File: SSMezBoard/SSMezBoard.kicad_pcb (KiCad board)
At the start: 2 copper layers, 2 parts, among them U1 DFRobot_DC_Controller

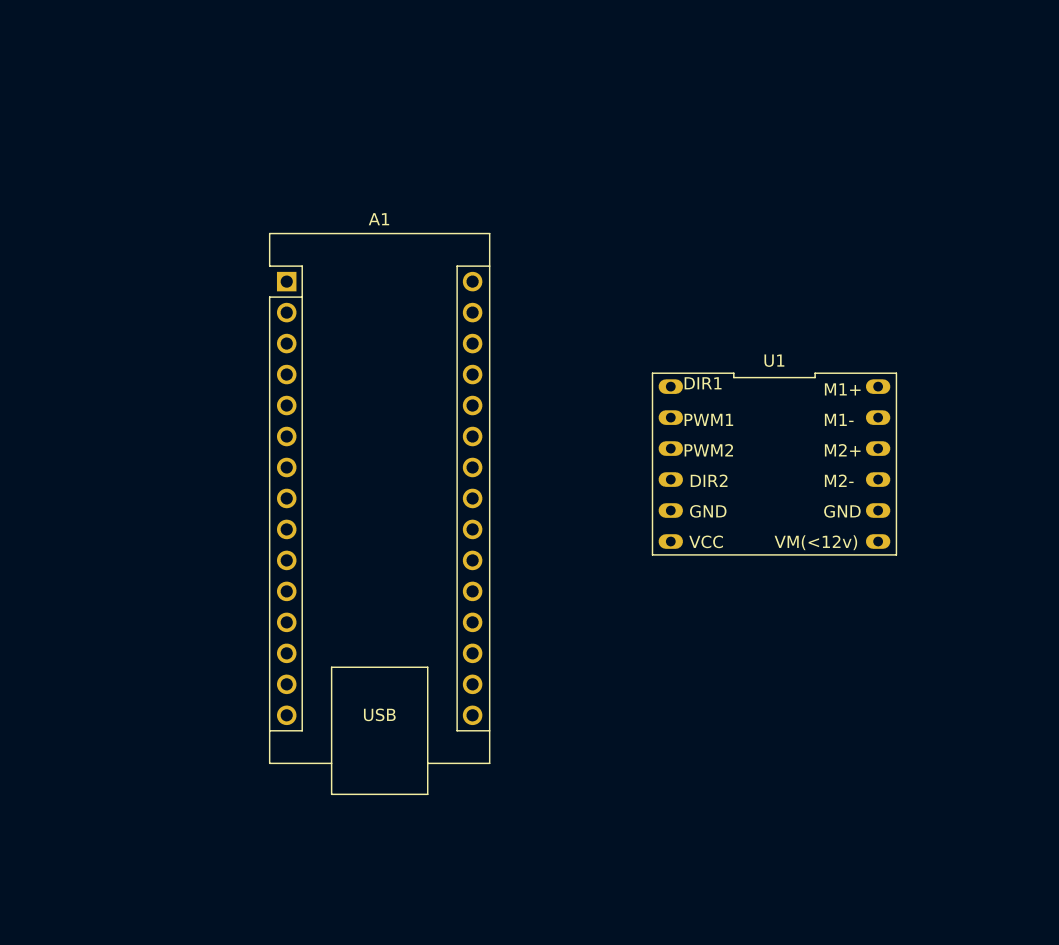
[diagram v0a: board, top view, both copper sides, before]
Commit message: Sort of ready for JLCPCB
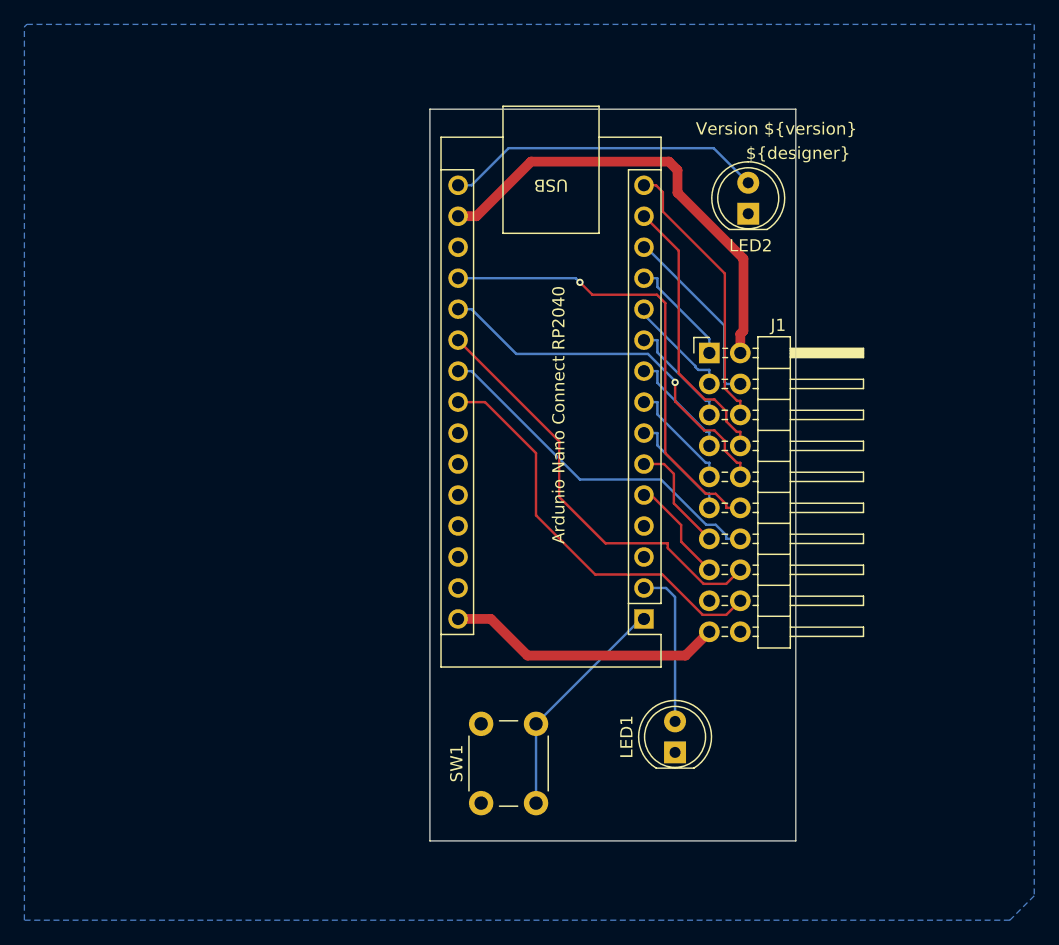
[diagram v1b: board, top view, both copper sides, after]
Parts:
- removed U1: DFRobot_DC_Controller, PBFootPrintLibrary:DFRobot_DC_Controller
- added J1: Conn_02x10_Odd_Even, Connector_PinHeader_2.54mm:PinHeader_2x10_P2.54mm_Horizontal, F.Cu at (162.9, 75.8)
- added LED1: LED, LED_THT:LED_D5.0mm, F.Cu at (160.1, 108.5)
- added LED2: LED, LED_THT:LED_D5.0mm, F.Cu at (166.1, 64.4)
- added SW1: TACT_SW, Button_Switch_THT:SW_PUSH_6mm, F.Cu at (144.2, 112.7)
- moved A1 40.3 mm to (157.6, 97.6), turned to 180 degrees
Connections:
- net Net-(A1-GND-Pad29) renamed GND
- A1 pad 1: unconnected-(A1-D1/TX-Pad1) -> Net-(A1-D1/TX)
- A1 pad 10: unconnected-(A1-D7-Pad10) -> RIGHT_ENC_B
- A1 pad 11: unconnected-(A1-D8-Pad11) -> LEFT_ENC_A
- A1 pad 12: unconnected-(A1-D9-Pad12) -> LEFT_ENC_B
- A1 pad 13: unconnected-(A1-D10/CS-Pad13) -> SENSOR_LED
- A1 pad 14: unconnected-(A1-D11/COPI-Pad14) -> GPIO_DIAG
- A1 pad 15: unconnected-(A1-D12/CIPO-Pad15) -> GPIO_FRONT
- A1 pad 16: unconnected-(A1-D13/SCK-Pad16) -> Net-(A1-D13/SCK)
- A1 pad 17: Net-(A1-3V3) -> Vcc
- A1 pad 19: unconnected-(A1-A0-Pad19) -> RIGHT_DIAG_ADC
- A1 pad 2: unconnected-(A1-D0/RX-Pad2) -> Net-(A1-D0/RX)
- A1 pad 20: unconnected-(A1-A1-Pad20) -> RIGHT_FRONT_ADC
- A1 pad 21: unconnected-(A1-A2-Pad21) -> LEFT_FRONT_ADC
- A1 pad 22: unconnected-(A1-A3-Pad22) -> LEFT_DIAG_ADC
- A1 pad 23: unconnected-(A1-SDA/A4-Pad23) -> GPIO12_D18
- A1 pad 30: unconnected-(A1-VIN-Pad30) -> Vbatt
- A1 pad 5: unconnected-(A1-D2-Pad5) -> RIGHT_Motor_PWM
- A1 pad 6: unconnected-(A1-D3-Pad6) -> LEFT_Motor_PWM
- A1 pad 7: unconnected-(A1-D4-Pad7) -> LEFT_Motor_Dir
- A1 pad 8: unconnected-(A1-D5-Pad8) -> RIGHT_Motor_Dir
- A1 pad 9: unconnected-(A1-D6-Pad9) -> RIGHT_ENC_A
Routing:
- net RIGHT_DIAG_ADC: track 0.00 -> 38.3 mm, vias 0 -> 1
- net Vcc: track 0.00 -> 37.5 mm
- net LEFT_FRONT_ADC: track 0.00 -> 34.8 mm
- net GPIO12_D18: track 0.00 -> 33.8 mm
- net RIGHT_FRONT_ADC: track 0.00 -> 31.0 mm, vias 0 -> 1
- net LEFT_DIAG_ADC: track 0.00 -> 29.0 mm
- net Net-(A1-D13/SCK): track 0.00 -> 26.2 mm
- net GPIO_FRONT: track 0.00 -> 22.8 mm
- net GPIO_DIAG: track 0.00 -> 22.7 mm
- net Vbatt: track 0.00 -> 22.7 mm
- net Net-(A1-D1/TX): track 0.00 -> 18.9 mm
- net SENSOR_LED: track 0.00 -> 15.3 mm
- net Net-(A1-D0/RX): track 0.00 -> 13.1 mm
- net LEFT_Motor_PWM: track 0.00 -> 9.32 mm
- net RIGHT_Motor_Dir: track 0.00 -> 9.16 mm
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- added copper zone on B.Cu, net GND
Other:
- board outline added: 30 x 60 mm
- board text added: "${designer}"
- board text added: "Ardunio Nano Connect RP2040"
- board text added: "Version ${version}"
